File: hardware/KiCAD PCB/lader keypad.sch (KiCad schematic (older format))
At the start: 13 parts, among them J1 CONNECTOR, SW1 Down, SW2 Left, SW3 Select, SW4 Up, SW5 Right

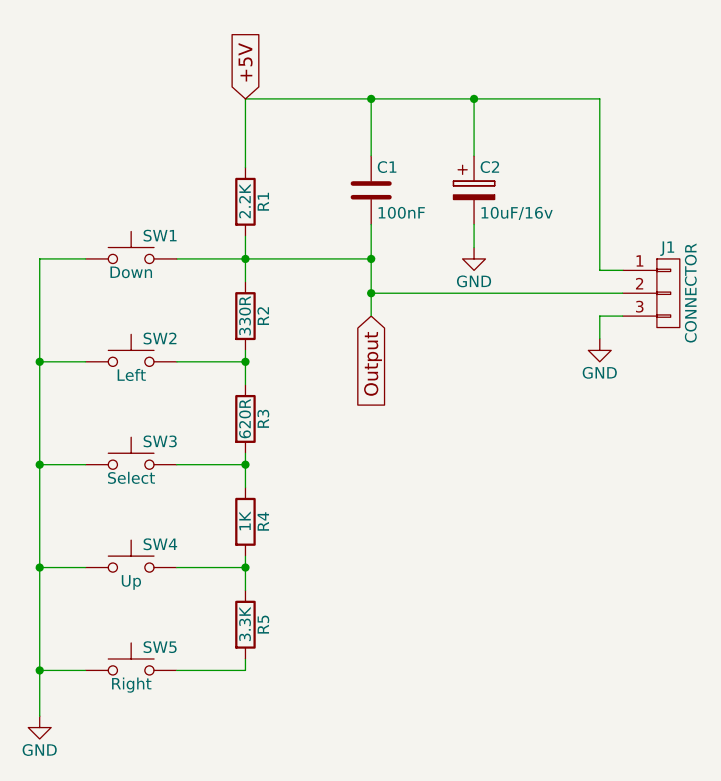
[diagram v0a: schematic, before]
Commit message: update hardware
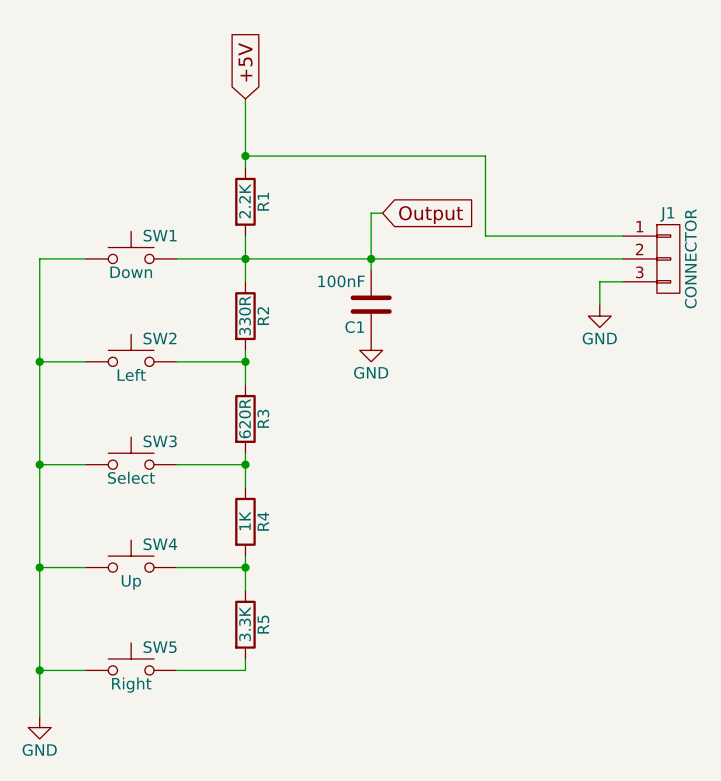
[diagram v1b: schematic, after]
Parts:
- removed C2: 10uF/16v, Capacitors_ThroughHole:CP_Radial_D6.3mm_P2.50mm, symbol CP
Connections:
- net +5V: no longer C1.1
- net GND: now also C1.1
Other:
- moved on the sheet: C1, J1
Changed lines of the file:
@@
 L C C1
 U 1 1 59309AF0
-P 6100 2050
-F 0 "C1" H 6125 2150 50  0000 L CNN
-F 1 "100nF" H 6125 1950 50  0000 L CNN
-F 2 "Capacitors_ThroughHole:C_Disc_D6.0mm_W2.5mm_P5.00mm" H 6138 1900 50  0001 C CNN
-F 3 "" H 6100 2050 50  0001 C CNN
-	1    6100 2050
-	1    0    0    -1
-$EndComp
-$Comp
-L CP C2
-U 1 1 59309B8B
-P 6550 2050
-F 0 "C2" H 6575 2150 50  0000 L CNN
-F 1 "10uF/16v" H 6575 1950 50  0000 L CNN
-F 2 "Capacitors_ThroughHole:CP_Radial_D6.3mm_P2.50mm" H 6588 1900 50  0001 C CNN
-F 3 "" H 6550 2050 50  0001 C CNN
-	1    6550 2050
-	1    0    0    -1
+P 6100 2550
+F 0 "C1" H 6125 2650 50  0000 L CNN
+F 1 "100nF" H 6125 2450 50  0000 L CNN
+F 2 "Capacitors_ThroughHole:C_Disc_D6.0mm_W2.5mm_P5.00mm" H 6138 2400 50  0001 C CNN
+F 3 "" H 6100 2550 50  0001 C CNN
+	1    6100 2550
+	-1   0    0    1
 $EndComp
 $Comp
@@
 $EndComp
 $Comp
-L GND #PWR02
-U 1 1 5930A314
-P 6550 2300
-F 0 "#PWR02" H 6550 2050 50  0001 C CNN
-F 1 "GND" H 6550 2150 50  0000 C CNN
-F 2 "" H 6550 2300 50  0001 C CNN
-F 3 "" H 6550 2300 50  0001 C CNN
-	1    6550 2300
+L CONN_01X03 J1
+U 1 1 5930A42E
+P 7400 2350
+F 0 "J1" H 7400 2550 50  0000 C CNN
+F 1 "CONNECTOR" V 7500 2350 50  0000 C CNN
+F 2 "Pin_Headers:Pin_Header_Straight_1x03_Pitch2.54mm" H 7400 2350 50  0001 C CNN
+F 3 "" H 7400 2350 50  0001 C CNN
+	1    7400 2350
 	1    0    0    -1
 $EndComp
 $Comp
-L CONN_01X03 J1
-U 1 1 5930A42E
-P 7400 2500
-F 0 "J1" H 7400 2700 50  0000 C CNN
-F 1 "CONNECTOR" V 7500 2500 50  0000 C CNN
-F 2 "Pin_Headers:Pin_Header_Straight_1x03_Pitch2.54mm" H 7400 2500 50  0001 C CNN
-F 3 "" H 7400 2500 50  0001 C CNN
-	1    7400 2500
+L GND #PWR02
+U 1 1 5930ABF0
+P 7100 2550
+F 0 "#PWR02" H 7100 2300 50  0001 C CNN
+F 1 "GND" H 7100 2400 50  0000 C CNN
+F 2 "" H 7100 2550 50  0001 C CNN
+F 3 "" H 7100 2550 50  0001 C CNN
+	1    7100 2550
 	1    0    0    -1
 $EndComp
-Wire Wire Line
-	6550 2200 6550 2300
-Wire Wire Line
-	6550 1900 6550 1650
-Wire Wire Line
-	5550 1650 7100 1650
+Text GLabel 5550 1650 1    60   Input ~ 0
++5V
+Text GLabel 6150 2150 2    60   Input ~ 0
+Output
 Wire Wire Line
 	5550 1650 5550 1950
-Wire Wire Line
-	6100 1900 6100 1650
-Connection ~ 6100 1650
-Wire Wire Line
-	6100 2200 6100 2600
-Wire Wire Line
-	6100 2350 5250 2350
 Wire Wire Line
 	5550 2250 5550 2450
@@
 	4850 4150 4650 4150
 Connection ~ 4650 4150
-Connection ~ 6550 1650
 Wire Wire Line
-	6100 2500 7200 2500
+	7200 2450 7100 2450
+Wire Wire Line
+	7100 2450 7100 2550
+Wire Wire Line
+	5550 1900 6600 1900
+Connection ~ 5550 1900
 Connection ~ 6100 2350
 $Comp
 L GND #PWR03
-U 1 1 5930ABF0
-P 7100 2700
-F 0 "#PWR03" H 7100 2450 50  0001 C CNN
-F 1 "GND" H 7100 2550 50  0000 C CNN
-F 2 "" H 7100 2700 50  0001 C CNN
-F 3 "" H 7100 2700 50  0001 C CNN
-	1    7100 2700
+U 1 1 59638407
+P 6100 2700
+F 0 "#PWR03" H 6100 2450 50  0001 C CNN
+F 1 "GND" H 6100 2550 50  0000 C CNN
+F 2 "" H 6100 2700 50  0001 C CNN
+F 3 "" H 6100 2700 50  0001 C CNN
+	1    6100 2700
 	1    0    0    -1
 $EndComp
 Wire Wire Line
-	7200 2600 7100 2600
+	5250 2350 7200 2350
 Wire Wire Line
-	7100 2600 7100 2700
+	7200 2250 6600 2250
 Wire Wire Line
-	7100 1650 7100 2400
+	6600 2250 6600 1900
 Wire Wire Line
-	7100 2400 7200 2400
-Text GLabel 5550 1650 1    60   Input ~ 0
-+5V
-Text GLabel 6100 2600 3    60   Input ~ 0
-Output
-Connection ~ 6100 2500
+	6150 2150 6100 2150
+Wire Wire Line
+	6100 2150 6100 2400
 $EndSCHEMATC
